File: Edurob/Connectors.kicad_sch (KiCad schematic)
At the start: 18 parts, among them J1 Conn_01x03_Male, J1 OLED, J12 Conn_01x06_Pin, J13 Conn_01x06_Pin, J14 Conn_01x06_Pin, J15 Conn_01x20_Pin, J16 Conn_01x20_Pin, J17 Conn_01x20_Pin, J18 Conn_01x20_Pin, J2 Conn_01x03_Male, J2 Conn_01x04_Pin, J3 Conn_01x04_Pin, J5 Conn_01x04_Pin, J7 Conn_01x06_Pin, J8 12402012E212A, J8 Conn_01x06_Pin

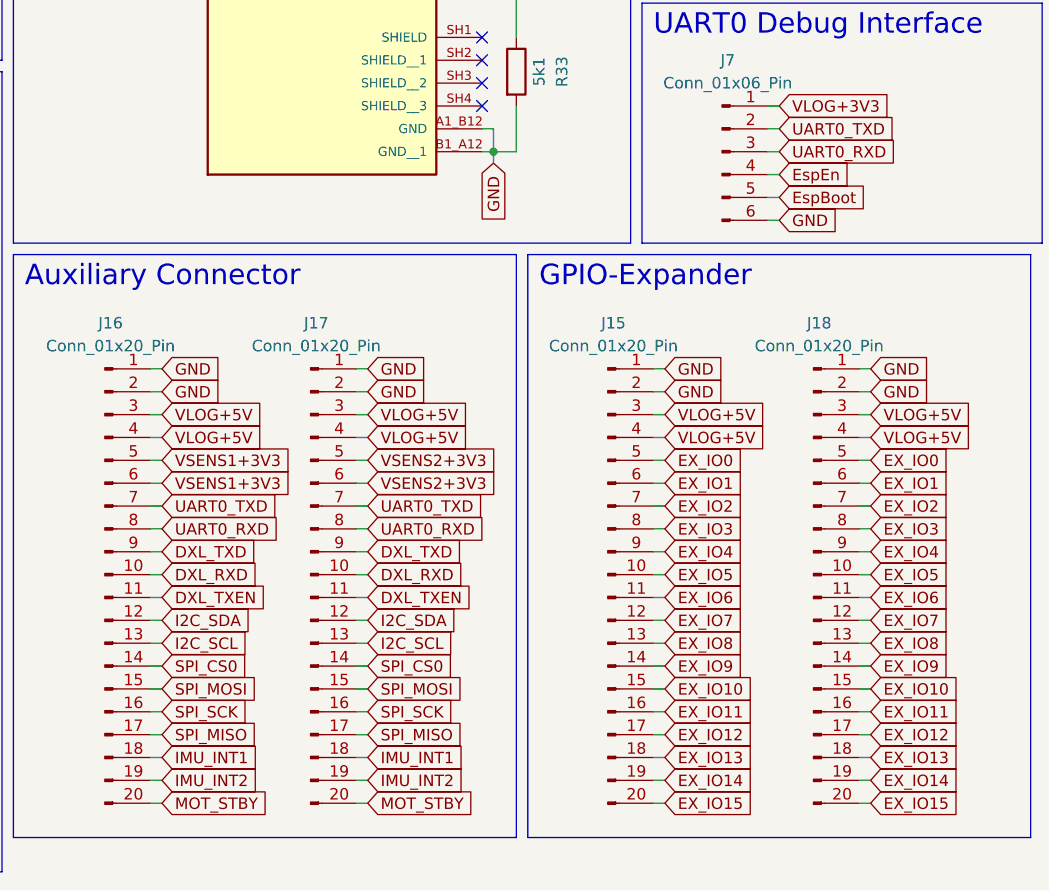
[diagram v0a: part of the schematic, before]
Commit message: Finalized part placement
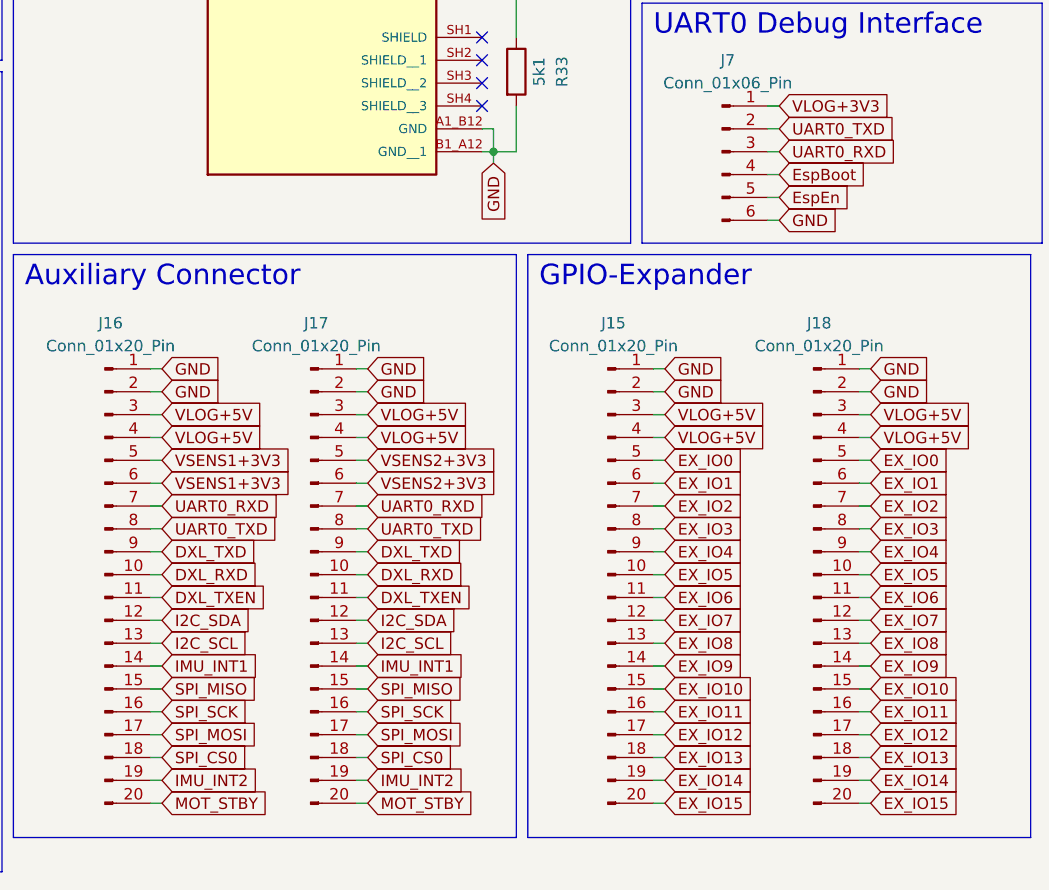
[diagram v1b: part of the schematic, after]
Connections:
- net EspBoot: now also J7.4 (Pin_4); no longer J7.5 (Pin_5)
- net EspEn: now also J7.5 (Pin_5); no longer J7.4 (Pin_4)
- net IMU_INT1: now also J16.14 (Pin_14), J17.14 (Pin_14); no longer J16.18 (Pin_18), J17.18 (Pin_18)
- net SPI_CS0: now also J16.18 (Pin_18), J17.18 (Pin_18); no longer J16.14 (Pin_14), J17.14 (Pin_14)
- net SPI_MISO: now also J16.15 (Pin_15), J17.15 (Pin_15); no longer J16.17 (Pin_17), J17.17 (Pin_17)
- net SPI_MOSI: now also J16.17 (Pin_17), J17.17 (Pin_17); no longer J16.15 (Pin_15), J17.15 (Pin_15)
- net UART0_RXD: now also J16.7 (Pin_7), J17.7 (Pin_7); no longer J16.8 (Pin_8), J17.8 (Pin_8)
- net UART0_TXD: now also J16.8 (Pin_8), J17.8 (Pin_8); no longer J16.7 (Pin_7), J17.7 (Pin_7)
